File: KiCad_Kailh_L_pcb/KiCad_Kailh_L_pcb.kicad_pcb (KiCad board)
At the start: 2 copper layers, 135.7 x 97.6 mm, 77 parts, among them J1 AudioJack3_SwitchTR, SW1 Esc, SW10 E, SW11 R, SW12 T, SW13 Ctrl, SW14 A, SW15 S, SW16 D, SW17 F, SW18 G, SW19 Shift, SW2 1, SW20 Z, SW21 X, SW22 C, SW23 V, SW24 6, SW25 Fn, SW26 Alt, SW27 Win, SW28 NoConv, SW29 Space, SW3 2, SW4 3, SW5 4, SW6 5, SW7 Tab, SW8 Q, SW9 W, U1 Sparkfun_Pro_Micro

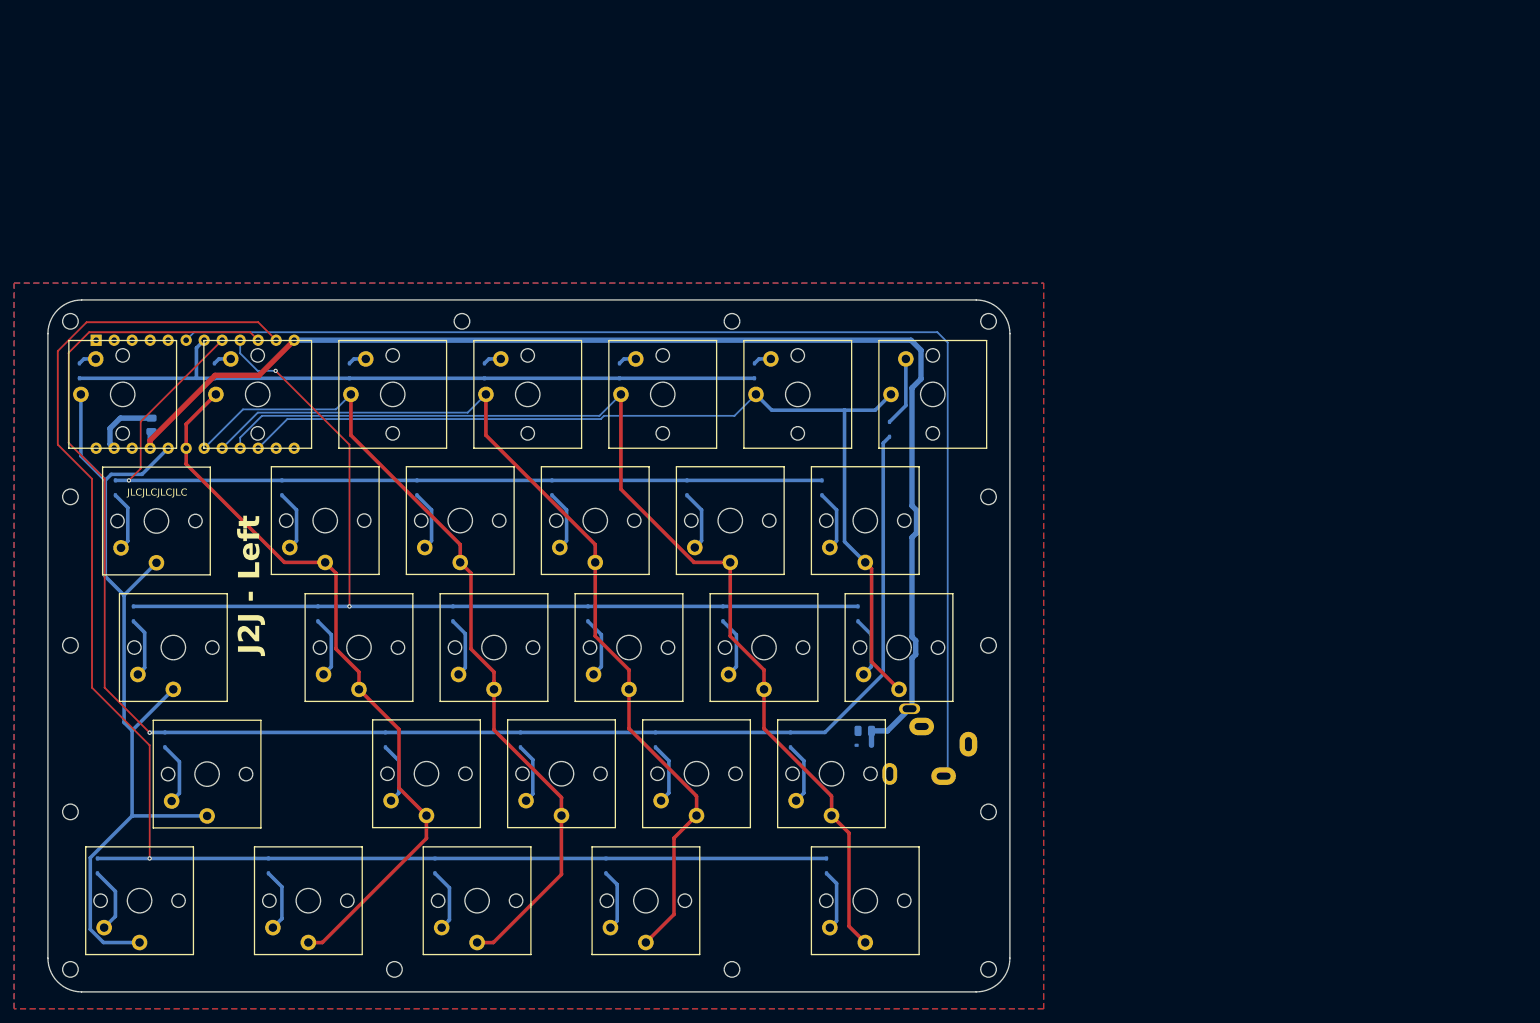
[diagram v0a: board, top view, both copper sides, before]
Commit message: refactor: 作り直し
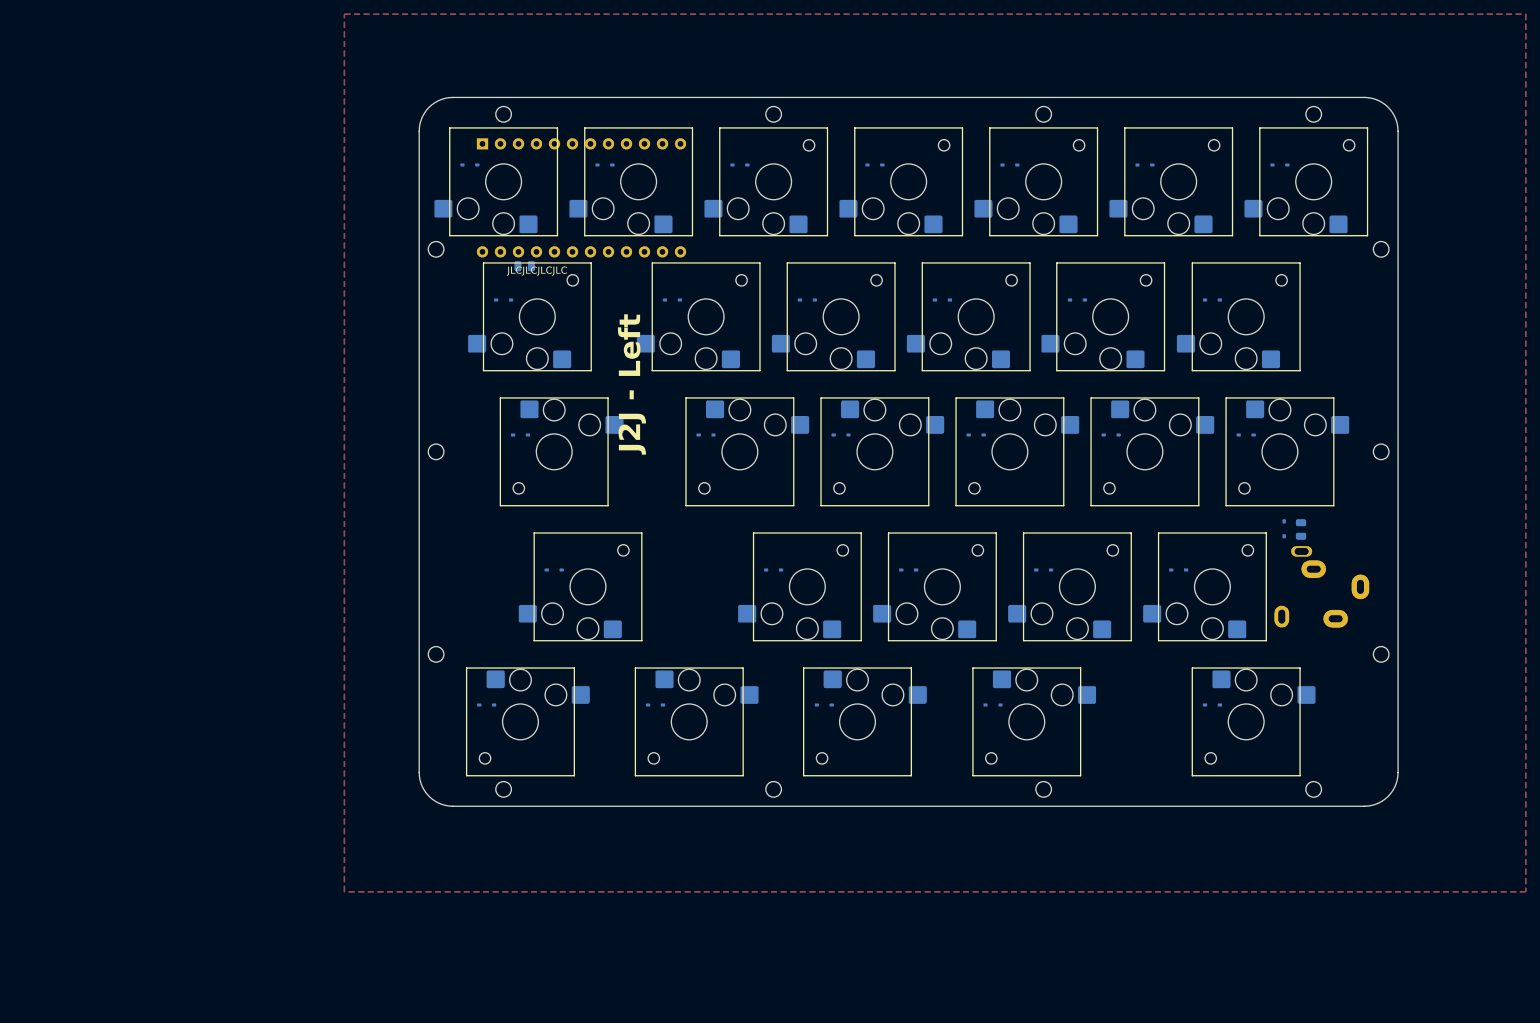
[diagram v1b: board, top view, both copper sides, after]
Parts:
- removed H1, H11, H5, H6: MountingHole_2.2mm_M2, MountingHole:MountingHole_2.2mm_M2
- added H2: MountingHole_2.2mm_M2, MountingHole:MountingHole_2.2mm_M2, F.Cu at (92.9, 142.9)
- added H2: MountingHole_2.2mm_M2, MountingHole:MountingHole_2.2mm_M2, F.Cu at (131.0, 142.9)
- added H2: MountingHole_2.2mm_M2, MountingHole:MountingHole_2.2mm_M2, F.Cu at (216.7, 95.2)
- added H2: MountingHole_2.2mm_M2, MountingHole:MountingHole_2.2mm_M2, F.Cu at (83.3, 95.2)
- SW1, SW10, SW11, SW12, SW14, SW15, SW16, SW17, SW18, SW2, SW20, SW21, SW22, SW23, SW24, SW3, SW4, SW5, SW6, SW8, SW9: footprint PCM_Switch_Keyboard_Kailh:SW_Kailh_Choc_V1_1.00u -> PCM_Switch_Keyboard_Hotswap_Kailh:SW_Hotswap_Kailh_Choc_V2_1.00u
- SW13: footprint PCM_Switch_Keyboard_Kailh:SW_Kailh_Choc_V1_1.75u -> PCM_Switch_Keyboard_Hotswap_Kailh:SW_Hotswap_Kailh_Choc_V2_1.75u
- SW19: footprint PCM_Switch_Keyboard_Kailh:SW_Kailh_Choc_V1_2.25u -> PCM_Switch_Keyboard_Hotswap_Kailh:SW_Hotswap_Kailh_Choc_V2_2.25u
- SW25, SW26, SW27, SW28: footprint PCM_Switch_Keyboard_Kailh:SW_Kailh_Choc_V1_1.25u -> PCM_Switch_Keyboard_Hotswap_Kailh:SW_Hotswap_Kailh_Choc_V2_1.25u
- SW29: footprint PCM_Switch_Keyboard_Kailh:SW_Kailh_Choc_V1_2.00u -> PCM_Switch_Keyboard_Hotswap_Kailh:SW_Hotswap_Kailh_Choc_V2_2.00u
- SW7: footprint PCM_Switch_Keyboard_Kailh:SW_Kailh_Choc_V1_1.50u -> PCM_Switch_Keyboard_Hotswap_Kailh:SW_Hotswap_Kailh_Choc_V2_1.50u
- moved H10 108.6 mm to (207.2, 47.6)
- moved H12 95.1 mm to (169.1, 142.9)
- moved H13 85.9 mm to (207.2, 142.9)
- moved H8 78.7 mm to (216.7, 66.7)
- moved H7 76.1 mm to (83.3, 66.7)
- moved H14 71.0 mm to (216.7, 123.8)
- moved C1 67.8 mm to (205.4, 106.2), turned to 90 degrees
- moved D30 66.7 mm to (203.0, 106.1), turned to 90 degrees
- moved D24 66.5 mm to (202.4, 54.8), turned to 0 degrees
- moved D1 62.3 mm to (88.1, 54.8), turned to 0 degrees
- moved D2 62.3 mm to (107.2, 54.8), turned to 0 degrees
- moved D3 62.3 mm to (126.2, 54.8), turned to 0 degrees
- moved D4 62.3 mm to (145.3, 54.8), turned to 0 degrees
- moved D5 62.3 mm to (164.3, 54.8), turned to 0 degrees
- moved D6 62.3 mm to (183.4, 54.8), turned to 0 degrees
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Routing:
- net Row3: track 227.5 -> 0.00 mm, vias 1 -> 0
- net Row4: track 213.4 -> 0.00 mm, vias 1 -> 0
- net +5V: track 179.7 -> 0.00 mm
- net SCL: track 169.9 -> 0.00 mm
- net Col4: track 152.4 -> 0.00 mm
- net Row2: track 147.7 -> 0.00 mm, vias 2 -> 0
- net Col5: track 136.9 -> 0.00 mm
- net Col3: track 133.0 -> 0.00 mm
- net Row1: track 124.9 -> 0.00 mm, vias 1 -> 0
- net Col0: track 124.7 -> 0.00 mm
- net Col2: track 120.9 -> 0.00 mm
- net Col1: track 104.5 -> 0.00 mm
- net Row0: track 101.1 -> 0.00 mm
- net Net-(D24-A): track 9.84 -> 0.00 mm
- net GND: track 9.48 -> 0.00 mm
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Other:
- board size 135.7 x 97.6 mm -> 138.1 x 100 mm
